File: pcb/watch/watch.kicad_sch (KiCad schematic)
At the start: 98 parts, among them U1 STM32G031K8Ux, U2 TLV74130PDQNR

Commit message: aa
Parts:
- R1, R2, R3, R4, R5: footprint footprints:R_0402_nosilk -> footprints:R_0402_nosilk_square
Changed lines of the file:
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@@
       (effects (font (size 1.27 1.27)) (justify left) hide)
     )
-    (property "Footprint" "footprints:R_0402_nosilk" (at 45.72 30.48 0)
+    (property "Footprint" "footprints:R_0402_nosilk_square" (at 45.72 30.48 0)
       (effects (font (size 1.27 1.27)) hide)
     )
@@
       (effects (font (size 1.27 1.27)) (justify left) hide)
     )
-    (property "Footprint" "footprints:R_0402_nosilk" (at 39.37 30.48 0)
+    (property "Footprint" "footprints:R_0402_nosilk_square" (at 39.37 30.48 0)
       (effects (font (size 1.27 1.27)) hide)
     )
@@
       (effects (font (size 1.27 1.27)) (justify left) hide)
     )
-    (property "Footprint" "footprints:R_0402_nosilk" (at 52.07 30.48 0)
+    (property "Footprint" "footprints:R_0402_nosilk_square" (at 52.07 30.48 0)
       (effects (font (size 1.27 1.27)) hide)
     )
@@
       (effects (font (size 1.27 1.27)) (justify left) hide)
     )
-    (property "Footprint" "footprints:R_0402_nosilk" (at 58.42 30.48 0)
+    (property "Footprint" "footprints:R_0402_nosilk_square" (at 58.42 30.48 0)
       (effects (font (size 1.27 1.27)) hide)
     )
@@
       (effects (font (size 1.27 1.27)) (justify left) hide)
     )
-    (property "Footprint" "footprints:R_0402_nosilk" (at 33.02 30.48 0)
-      (effects (font (size 1.27 1.27)) hide)
-    )
+    (property "Footprint" "footprints:R_0402_nosilk_square" (at 33.02 30.48 0)
+      (effects (font (size 1.27 1.27)) hide)
+    )

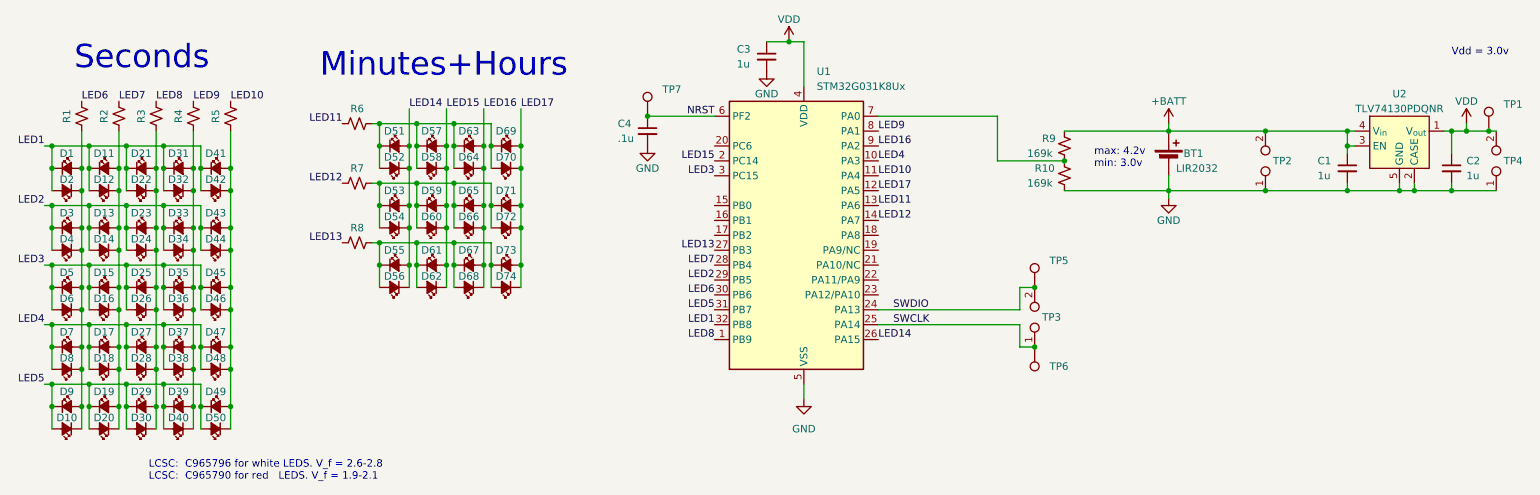
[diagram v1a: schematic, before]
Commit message: eee
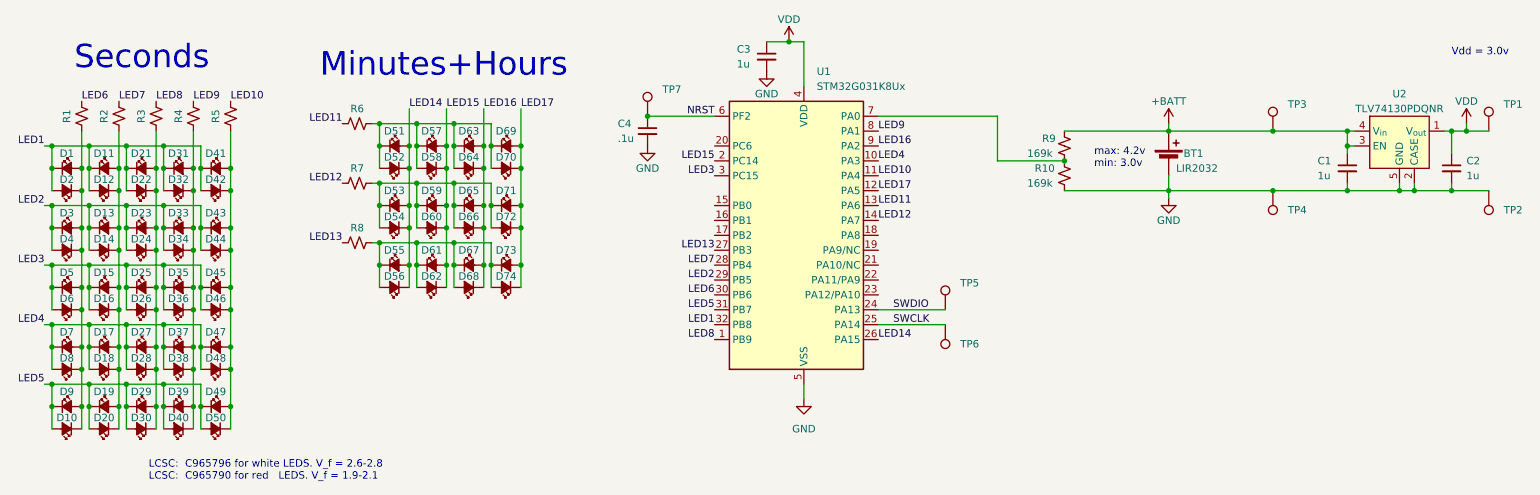
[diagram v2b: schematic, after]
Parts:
- removed TP2, TP3, TP4: TestPoint_2Pole, footprints:tesptoint_tiny, symbol Connector:TestPoint_2Pole
- added TP2, TP4: TestPoint, footprints:testpoint_better_square, symbol Connector:TestPoint
- added TP3: TestPoint, footprints:testpoint_better, symbol Connector:TestPoint
- D10, D12, D13, D14, D15, D16, D17, D18, D19, D2, D20, D22, D23, D24, D25, D26, D27, D28, D29, D3, D30, D32, D33, D34, D35, D36, D37, D38, D39, D4, D40, D42, D43, D44, D45, D46, D47, D48, D49, D5, D50, D6, D7, D8, D9: footprint LED_SMD:LED_0402_1005Metric -> footprints:LED_0402_nosilk
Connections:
- net +BATT: now also TP3.1
- net GND: now also TP2.1, TP4.1
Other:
- moved on the sheet: TP5, TP6
